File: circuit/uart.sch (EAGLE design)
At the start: 2 parts

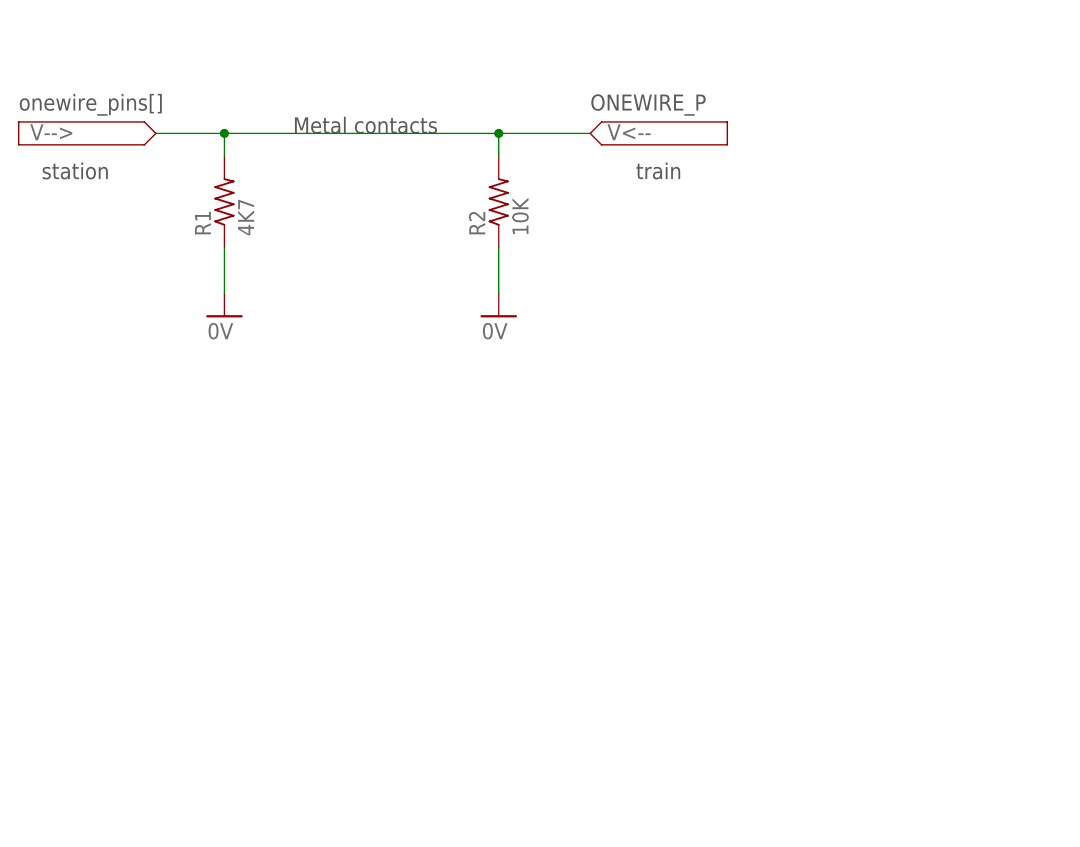
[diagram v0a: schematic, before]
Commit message: New circuit
Hopefully the final
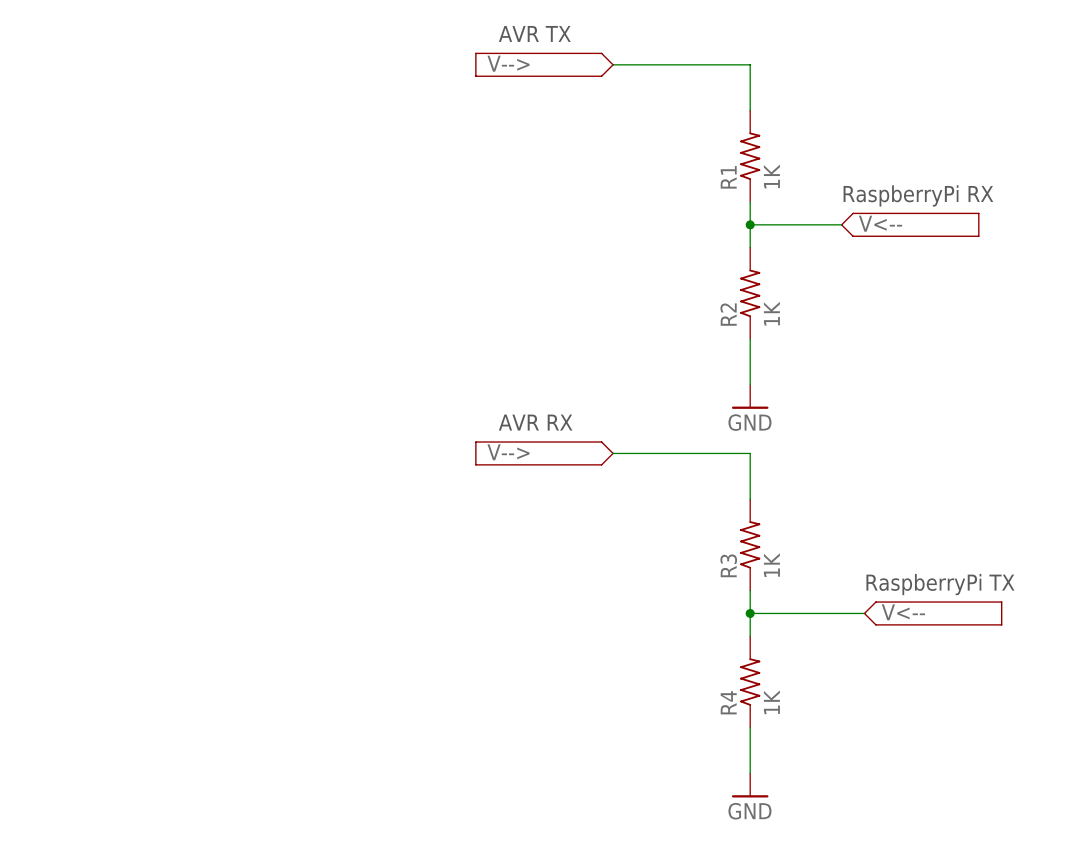
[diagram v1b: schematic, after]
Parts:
- added R3, R4: 1K, resistor:R-US_0204/5
- R1: value 4K7 -> 1K; device resistor:R-US_0204/7 -> resistor:R-US_0204/5
- R2: value 10K -> 1K; device resistor:R-US_0204/7 -> resistor:R-US_0204/5
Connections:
- removed net 0V: R1.1, R2.1
- new net GND: R2.1, R4.1
- new net N$2: R1.1, R2.2
- new net N$3: R3.2
- new net N$4: R3.1, R4.2
- net N$1: no longer R2.2
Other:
- note added: "AVR RX"
- note added: "AVR TX"
- note added: "RaspberryPi RX"
- note added: "RaspberryPi TX"
- note removed: "Metal contacts"
- note removed: "ONEWIRE_P"
- note removed: "onewire_pins[]"
- note removed: "station"
- note removed: "train"
- moved on the sheet: R1, R2
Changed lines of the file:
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@@
 </classes>
 <parts>
-<part name="R1" library="resistor" deviceset="R-US_" device="0204/7" value="4K7"/>
-<part name="R2" library="resistor" deviceset="R-US_" device="0204/7" value="10K"/>
-<part name="GND1" library="supply1" deviceset="0V" device=""/>
-<part name="GND2" library="supply1" deviceset="0V" device=""/>
+<part name="R1" library="resistor" deviceset="R-US_" device="0204/5" value="1K"/>
+<part name="R2" library="resistor" deviceset="R-US_" device="0204/5" value="1K"/>
+<part name="R3" library="resistor" deviceset="R-US_" device="0204/5" value="1K"/>
+<part name="R4" library="resistor" deviceset="R-US_" device="0204/5" value="1K"/>
+<part name="GND1" library="supply1" deviceset="GND" device=""/>
+<part name="GND2" library="supply1" deviceset="GND" device=""/>
 <part name="SUPPLY1" library="supply2" deviceset="V--&gt;" device=""/>
-<part name="SUPPLY2" library="supply2" deviceset="V&lt;--" device=""/>
+<part name="SUPPLY2" library="supply2" deviceset="V--&gt;" device=""/>
+<part name="SUPPLY3" library="supply2" deviceset="V&lt;--" device=""/>
+<part name="SUPPLY4" library="supply2" deviceset="V&lt;--" device=""/>
 </parts>
 <sheets>
 <sheet>
 <plain>
-<text x="33.02" y="68.58" size="1.778" layer="97">ONEWIRE_P</text>
-<text x="-30.48" y="68.58" size="1.778" layer="97">onewire_pins[]</text>
-<text x="0" y="66.04" size="1.778" layer="97">Metal contacts</text>
-<text x="-27.94" y="60.96" size="1.778" layer="97">station</text>
-<text x="38.1" y="60.96" size="1.778" layer="97">train</text>
+<text x="22.86" y="76.2" size="1.778" layer="97">AVR TX</text>
+<text x="22.86" y="33.02" size="1.778" layer="97">AVR RX</text>
+<text x="63.5" y="15.24" size="1.778" layer="97">RaspberryPi TX</text>
+<text x="60.96" y="58.42" size="1.778" layer="97">RaspberryPi RX</text>
 </plain>
 <instances>
-<instance part="R1" gate="G$1" x="-7.62" y="58.42" rot="R90"/>
-<instance part="R2" gate="G$1" x="22.86" y="58.42" rot="R90"/>
-<instance part="GND1" gate="1" x="-7.62" y="45.72"/>
-<instance part="GND2" gate="1" x="22.86" y="45.72"/>
-<instance part="SUPPLY1" gate="G$1" x="-30.48" y="66.04"/>
-<instance part="SUPPLY2" gate="G$1" x="48.26" y="66.04"/>
+<instance part="R1" gate="G$1" x="50.8" y="63.5" rot="R90"/>
+<instance part="R2" gate="G$1" x="50.8" y="48.26" rot="R90"/>
+<instance part="R3" gate="G$1" x="50.8" y="20.32" rot="R90"/>
+<instance part="R4" gate="G$1" x="50.8" y="5.08" rot="R90"/>
+<instance part="GND1" gate="1" x="50.8" y="35.56"/>
+<instance part="GND2" gate="1" x="50.8" y="-7.62"/>
+<instance part="SUPPLY1" gate="G$1" x="20.32" y="73.66"/>
+<instance part="SUPPLY2" gate="G$1" x="20.32" y="30.48"/>
+<instance part="SUPPLY3" gate="G$1" x="78.74" y="12.7"/>
+<instance part="SUPPLY4" gate="G$1" x="76.2" y="55.88"/>
 </instances>
 <busses>
@@
 <net name="N$1" class="0">
 <segment>
-<wire x1="-15.24" y1="66.04" x2="-7.62" y2="66.04" width="0.1524" layer="91"/>
 <pinref part="R1" gate="G$1" pin="2"/>
-<wire x1="33.02" y1="66.04" x2="22.86" y2="66.04" width="0.1524" layer="91"/>
-<wire x1="22.86" y1="66.04" x2="-7.62" y2="66.04" width="0.1524" layer="91"/>
-<wire x1="-7.62" y1="66.04" x2="-7.62" y2="63.5" width="0.1524" layer="91"/>
-<pinref part="R2" gate="G$1" pin="2"/>
-<wire x1="22.86" y1="66.04" x2="22.86" y2="63.5" width="0.1524" layer="91"/>
-<junction x="22.86" y="66.04"/>
-<junction x="-7.62" y="66.04"/>
+<wire x1="35.56" y1="73.66" x2="50.8" y2="73.66" width="0.1524" layer="91"/>
+<wire x1="50.8" y1="73.66" x2="50.8" y2="68.58" width="0.1524" layer="91"/>
 </segment>
 </net>
-<net name="0V" class="0">
+<net name="N$2" class="0">
 <segment>
 <pinref part="R1" gate="G$1" pin="1"/>
-<pinref part="GND1" gate="1" pin="0V"/>
-<wire x1="-7.62" y1="53.34" x2="-7.62" y2="48.26" width="0.1524" layer="91"/>
+<pinref part="R2" gate="G$1" pin="2"/>
+<wire x1="50.8" y1="58.42" x2="50.8" y2="55.88" width="0.1524" layer="91"/>
+<wire x1="50.8" y1="55.88" x2="50.8" y2="53.34" width="0.1524" layer="91"/>
+<wire x1="60.96" y1="55.88" x2="50.8" y2="55.88" width="0.1524" layer="91"/>
+<junction x="50.8" y="55.88"/>
+</segment>
+</net>
+<net name="GND" class="0">
+<segment>
+<pinref part="R2" gate="G$1" pin="1"/>
+<pinref part="GND1" gate="1" pin="GND"/>
+<wire x1="50.8" y1="43.18" x2="50.8" y2="38.1" width="0.1524" layer="91"/>
 </segment>
 <segment>
-<pinref part="R2" gate="G$1" pin="1"/>
-<pinref part="GND2" gate="1" pin="0V"/>
-<wire x1="22.86" y1="53.34" x2="22.86" y2="48.26" width="0.1524" layer="91"/>
+<pinref part="R4" gate="G$1" pin="1"/>
+<pinref part="GND2" gate="1" pin="GND"/>
+<wire x1="50.8" y1="0" x2="50.8" y2="-5.08" width="0.1524" layer="91"/>
 </segment>
 </net>
+<net name="N$3" class="0">
+<segment>
+<pinref part="R3" gate="G$1" pin="2"/>
+<wire x1="50.8" y1="25.4" x2="50.8" y2="30.48" width="0.1524" layer="91"/>
+<wire x1="50.8" y1="30.48" x2="35.56" y2="30.48" width="0.1524" layer="91"/>
+</segment>
+</net>
+<net name="N$4" class="0">
+<segment>
+<pinref part="R3" gate="G$1" pin="1"/>
+<pinref part="R4" gate="G$1" pin="2"/>
+<wire x1="50.8" y1="15.24" x2="50.8" y2="12.7" width="0.1524" layer="91"/>
+<wire x1="50.8" y1="12.7" x2="50.8" y2="10.16" width="0.1524" layer="91"/>
+<wire x1="63.5" y1="12.7" x2="50.8" y2="12.7" width="0.1524" layer="91"/>
+<junction x="50.8" y="12.7"/>
+</segment>
+</net>
